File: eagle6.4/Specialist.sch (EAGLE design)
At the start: 110 parts, among them X1 SCART-F

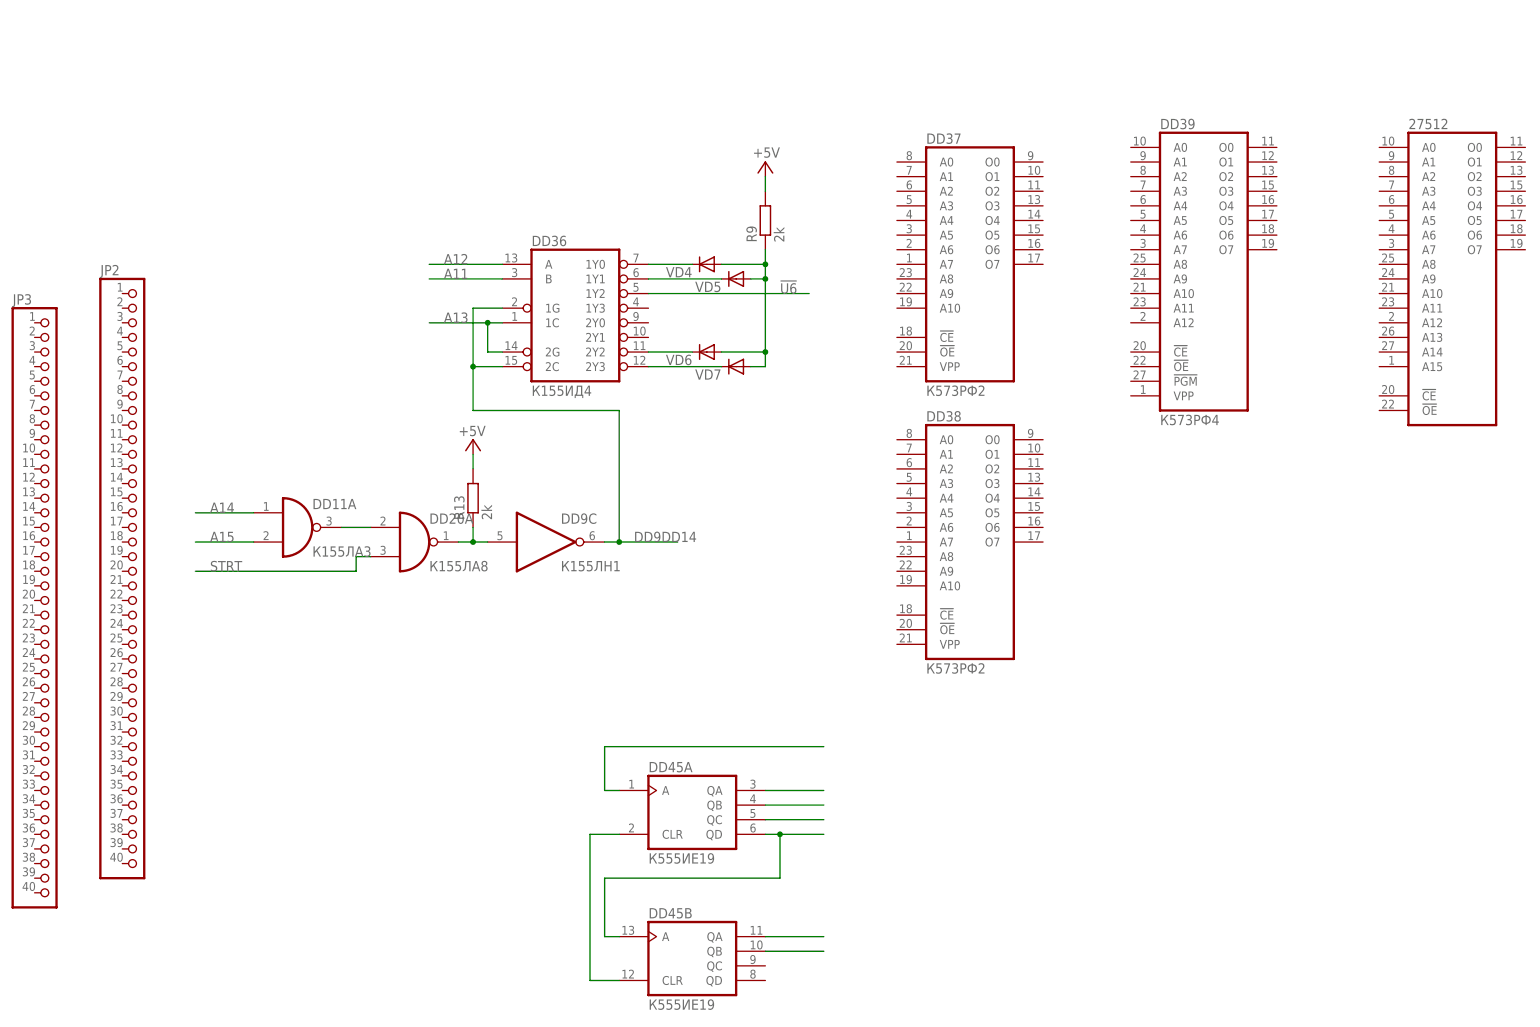
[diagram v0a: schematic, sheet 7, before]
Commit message: .
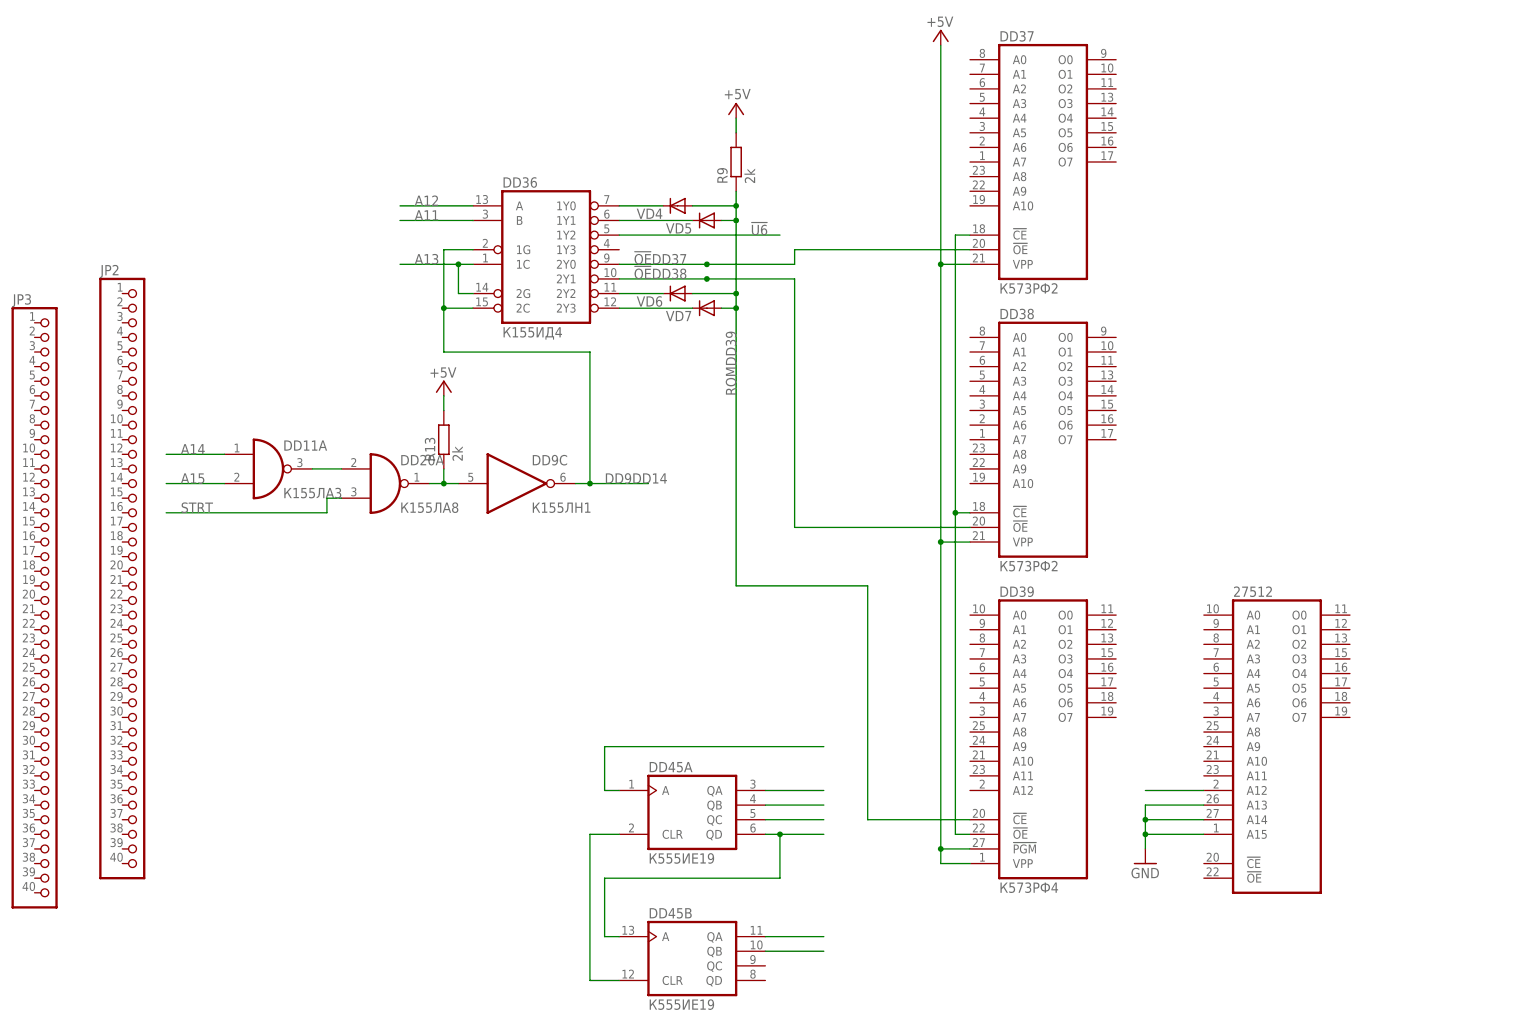
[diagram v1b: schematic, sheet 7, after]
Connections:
- new net !OE!DD37: DD36A.2Y0, DD37A.!OE
- new net !OE!DD38: DD36A.2Y1, DD38A.!OE
- new net N$33: DD37A.!CE, DD38A.!CE, DD39A.!OE
- new net ROMDD39: DD39A.!CE, R9.1, VD4.A, VD5.A, VD6.A, VD7.A
- net +5V: now also DD37A.VPP, DD38A.VPP, DD39A.!PGM, DD39A.VPP
- net GND: now also 27512A.A13, 27512A.A14, 27512A.A15
- net N$18: now also 27512A.A12; no longer R9.1, VD4.A, VD5.A, VD6.A, VD7.A
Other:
- note added: "dd37 dd38 dd39 09 oedd37 1 0 1 10 oedd38 1 1 0 d romdd39 1 1 1"
- note added: "test norm sd a13 0 0 1 a14 0 0 0 a15 0 0 0"
- moved on the sheet: 27512, DD11A, DD20A, DD36, DD37, DD38, DD39, DD9C, R13, R9, VD4, VD5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
